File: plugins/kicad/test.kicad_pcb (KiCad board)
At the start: 2 copper layers, 172.7 x 40.6 mm, 2 parts

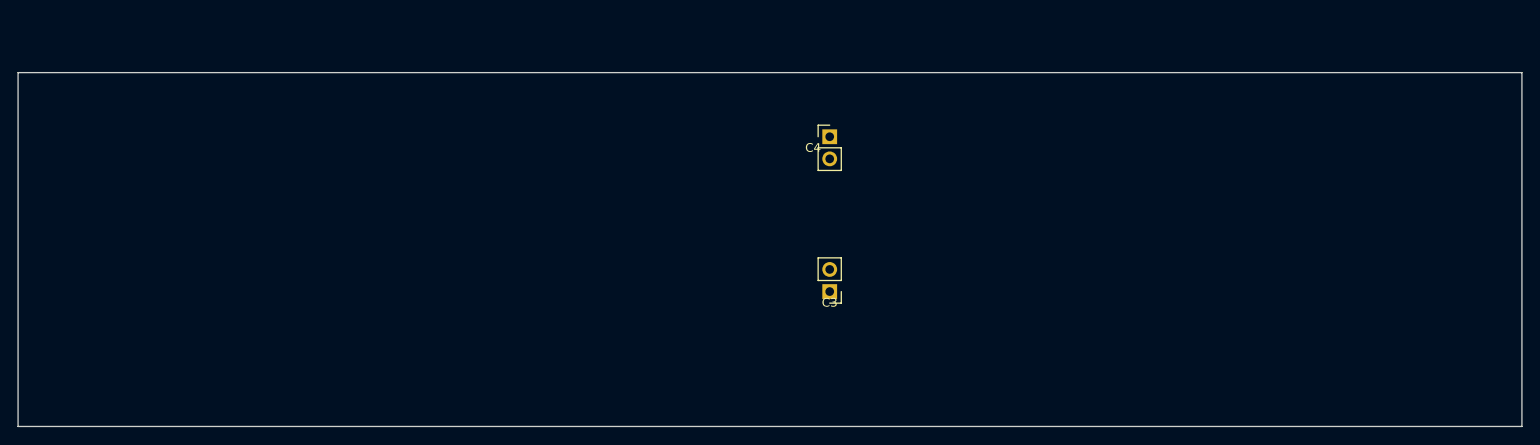
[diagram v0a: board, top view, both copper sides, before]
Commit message: perfectGPT
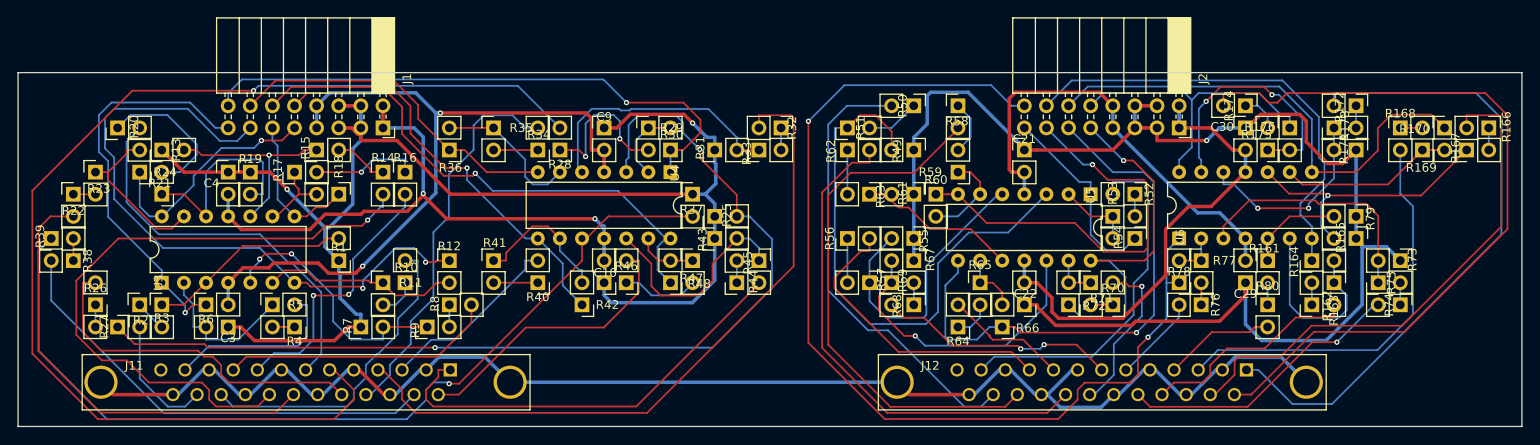
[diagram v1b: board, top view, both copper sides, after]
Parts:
- added C10: 100n, Connector_PinHeader_2.54mm:PinHeader_1x02_P2.54mm_Vertical, F.Cu at (134.6, 215.3)
- added C21: 100n, Connector_PinHeader_2.54mm:PinHeader_1x02_P2.54mm_Vertical, F.Cu at (182.9, 200.0)
- added C22: 100n, Connector_PinHeader_2.54mm:PinHeader_1x02_P2.54mm_Vertical, F.Cu at (182.9, 217.8)
- added C29: 100n, Connector_PinHeader_2.54mm:PinHeader_1x02_P2.54mm_Vertical, F.Cu at (208.3, 215.3)
- added C30: 100n, Connector_PinHeader_2.54mm:PinHeader_1x02_P2.54mm_Vertical, F.Cu at (208.3, 197.5)
- added C9: 100n, Connector_PinHeader_2.54mm:PinHeader_1x02_P2.54mm_Vertical, F.Cu at (134.6, 197.5)
- added J1: CONN_02X08, Connector_PinSocket_2.54mm:PinSocket_2x08_P2.54mm_Horizontal, F.Cu at (109.2, 197.5)
- added J11: DB25_FEMALE, anatalpretty:DB25FD, F.Cu at (100.3, 226.7)
- added J12: DB25_FEMALE, anatalpretty:DB25FD, F.Cu at (191.8, 226.7)
- added J2: CONN_02X08, Connector_PinSocket_2.54mm:PinSocket_2x08_P2.54mm_Horizontal, F.Cu at (200.7, 197.5)
- added R1: 10k, Connector_PinHeader_2.54mm:PinHeader_1x02_P2.54mm_Vertical, F.Cu at (104.1, 212.7)
- added R10: 10k, Connector_PinHeader_2.54mm:PinHeader_1x02_P2.54mm_Vertical, F.Cu at (111.8, 215.3)
- added R11: 10k, Connector_PinHeader_2.54mm:PinHeader_1x02_P2.54mm_Vertical, F.Cu at (109.2, 215.3)
- added R12: 10k, Connector_PinHeader_2.54mm:PinHeader_1x02_P2.54mm_Vertical, F.Cu at (116.8, 212.7)
- added R13: 10k, Connector_PinHeader_2.54mm:PinHeader_1x02_P2.54mm_Vertical, F.Cu at (83.8, 200.0)
- added R14: 10k, Connector_PinHeader_2.54mm:PinHeader_1x02_P2.54mm_Vertical, F.Cu at (109.2, 202.6)
- added R15: 10k, Connector_PinHeader_2.54mm:PinHeader_1x02_P2.54mm_Vertical, F.Cu at (101.6, 200.0)
- added R16: 10k, Connector_PinHeader_2.54mm:PinHeader_1x02_P2.54mm_Vertical, F.Cu at (111.8, 202.6)
- added R161: 10k, Connector_PinHeader_2.54mm:PinHeader_1x02_P2.54mm_Vertical, F.Cu at (210.8, 212.7)
- added R162: 10k, Connector_PinHeader_2.54mm:PinHeader_1x02_P2.54mm_Vertical, F.Cu at (215.9, 217.8)
- added R163: 10k, Connector_PinHeader_2.54mm:PinHeader_1x02_P2.54mm_Vertical, F.Cu at (218.4, 215.3)
- added R164: 10k, Connector_PinHeader_2.54mm:PinHeader_1x02_P2.54mm_Vertical, F.Cu at (215.9, 212.7)
- added R165: 10k, Connector_PinHeader_2.54mm:PinHeader_1x02_P2.54mm_Vertical, F.Cu at (221.0, 210.2)
- added R166: 10k, Connector_PinHeader_2.54mm:PinHeader_1x02_P2.54mm_Vertical, F.Cu at (236.2, 197.5)
- added R167: 10k, Connector_PinHeader_2.54mm:PinHeader_1x02_P2.54mm_Vertical, F.Cu at (233.7, 200.0)
- added R168: 10k, Connector_PinHeader_2.54mm:PinHeader_1x02_P2.54mm_Vertical, F.Cu at (226.1, 197.5)
- added R169: 10k, Connector_PinHeader_2.54mm:PinHeader_1x02_P2.54mm_Vertical, F.Cu at (228.6, 200.0)
- added R17: 10k, Connector_PinHeader_2.54mm:PinHeader_1x02_P2.54mm_Vertical, F.Cu at (99.1, 202.6)
- added R170: 10k, Connector_PinHeader_2.54mm:PinHeader_1x02_P2.54mm_Vertical, F.Cu at (231.1, 197.5)
- added R171: 10k, Connector_PinHeader_2.54mm:PinHeader_1x02_P2.54mm_Vertical, F.Cu at (221.0, 200.0)
- added R172: 10k, Connector_PinHeader_2.54mm:PinHeader_1x02_P2.54mm_Vertical, F.Cu at (221.0, 194.9)
- added R173: 10k, Connector_PinHeader_2.54mm:PinHeader_1x02_P2.54mm_Vertical, F.Cu at (218.4, 197.5)
- added R174: 10k, Connector_PinHeader_2.54mm:PinHeader_1x02_P2.54mm_Vertical, F.Cu at (208.3, 194.9)
- added R175: 10k, Connector_PinHeader_2.54mm:PinHeader_1x02_P2.54mm_Vertical, F.Cu at (210.8, 200.0)
- added R176: 10k, Connector_PinHeader_2.54mm:PinHeader_1x02_P2.54mm_Vertical, F.Cu at (213.4, 197.5)
- added R18: 10k, Connector_PinHeader_2.54mm:PinHeader_1x02_P2.54mm_Vertical, F.Cu at (104.1, 205.1)
- added R19: 10k, Connector_PinHeader_2.54mm:PinHeader_1x02_P2.54mm_Vertical, F.Cu at (94.0, 202.6)
- added R2: 10k, Connector_PinHeader_2.54mm:PinHeader_1x02_P2.54mm_Vertical, F.Cu at (81.3, 217.8)
- added R20: 10k, Connector_PinHeader_2.54mm:PinHeader_1x02_P2.54mm_Vertical, F.Cu at (78.7, 197.5)
- added R21: 10k, Connector_PinHeader_2.54mm:PinHeader_1x02_P2.54mm_Vertical, F.Cu at (83.8, 205.1)
- added R22: 10k, Connector_PinHeader_2.54mm:PinHeader_1x02_P2.54mm_Vertical, F.Cu at (73.7, 205.1)
- added R23: 10k, Connector_PinHeader_2.54mm:PinHeader_1x02_P2.54mm_Vertical, F.Cu at (76.2, 202.6)
- added R24: 10k, Connector_PinHeader_2.54mm:PinHeader_1x02_P2.54mm_Vertical, F.Cu at (81.3, 202.6)
- added R25: 10k, Connector_PinHeader_2.54mm:PinHeader_1x02_P2.54mm_Vertical, F.Cu at (147.3, 207.6)
- added R26: 10k, Connector_PinHeader_2.54mm:PinHeader_1x02_P2.54mm_Vertical, F.Cu at (76.2, 217.8)
- added R27: 10k, Connector_PinHeader_2.54mm:PinHeader_1x02_P2.54mm_Vertical, F.Cu at (78.7, 220.3)
- added R28: 10k, Connector_PinHeader_2.54mm:PinHeader_1x02_P2.54mm_Vertical, F.Cu at (129.5, 200.0)
- added R29: 10k, Connector_PinHeader_2.54mm:PinHeader_1x02_P2.54mm_Vertical, F.Cu at (139.7, 197.5)
- added R3: 10k, Connector_PinHeader_2.54mm:PinHeader_1x02_P2.54mm_Vertical, F.Cu at (83.8, 217.8)
- added R30: 10k, Connector_PinHeader_2.54mm:PinHeader_1x02_P2.54mm_Vertical, F.Cu at (142.2, 200.0)
- added R31: 10k, Connector_PinHeader_2.54mm:PinHeader_1x02_P2.54mm_Vertical, F.Cu at (147.3, 200.0)
- added R32: 10k, Connector_PinHeader_2.54mm:PinHeader_1x02_P2.54mm_Vertical, F.Cu at (154.9, 197.5)
- added R33: 10k, Connector_PinHeader_2.54mm:PinHeader_1x02_P2.54mm_Vertical, F.Cu at (152.4, 200.0)
- added R34: 10k, Connector_PinHeader_2.54mm:PinHeader_1x02_P2.54mm_Vertical, F.Cu at (127.0, 200.0)
- added R35: 10k, Connector_PinHeader_2.54mm:PinHeader_1x02_P2.54mm_Vertical, F.Cu at (121.9, 197.5)
- added R36: 10k, Connector_PinHeader_2.54mm:PinHeader_1x02_P2.54mm_Vertical, F.Cu at (116.8, 200.0)
- added R37: 10k, Connector_PinHeader_2.54mm:PinHeader_1x02_P2.54mm_Vertical, F.Cu at (144.8, 205.1)
- added R38: 10k, Connector_PinHeader_2.54mm:PinHeader_1x02_P2.54mm_Vertical, F.Cu at (73.7, 212.7)
- added R39: 10k, Connector_PinHeader_2.54mm:PinHeader_1x02_P2.54mm_Vertical, F.Cu at (71.1, 210.2)
- added R4: 10k, Connector_PinHeader_2.54mm:PinHeader_1x02_P2.54mm_Vertical, F.Cu at (99.1, 220.3)
- added R40: 10k, Connector_PinHeader_2.54mm:PinHeader_1x02_P2.54mm_Vertical, F.Cu at (127.0, 215.3)
- added R41: 10k, Connector_PinHeader_2.54mm:PinHeader_1x02_P2.54mm_Vertical, F.Cu at (121.9, 212.7)
- added R42: 10k, Connector_PinHeader_2.54mm:PinHeader_1x02_P2.54mm_Vertical, F.Cu at (132.1, 217.8)
- added R43: 10k, Connector_PinHeader_2.54mm:PinHeader_1x02_P2.54mm_Vertical, F.Cu at (147.3, 210.2)
- added R44: 10k, Connector_PinHeader_2.54mm:PinHeader_1x02_P2.54mm_Vertical, F.Cu at (149.9, 215.3)
- added R45: 10k, Connector_PinHeader_2.54mm:PinHeader_1x02_P2.54mm_Vertical, F.Cu at (152.4, 212.7)
- added R46: 10k, Connector_PinHeader_2.54mm:PinHeader_1x02_P2.54mm_Vertical, F.Cu at (137.2, 215.3)
- added R47: 10k, Connector_PinHeader_2.54mm:PinHeader_1x02_P2.54mm_Vertical, F.Cu at (144.8, 212.7)
- added R48: 10k, Connector_PinHeader_2.54mm:PinHeader_1x02_P2.54mm_Vertical, F.Cu at (142.2, 215.3)
- added R49: 10k, Connector_PinHeader_2.54mm:PinHeader_1x02_P2.54mm_Vertical, F.Cu at (170.2, 200.0)
- added R5: 10k, Connector_PinHeader_2.54mm:PinHeader_1x02_P2.54mm_Vertical, F.Cu at (96.5, 217.8)
- added R50: 10k, Connector_PinHeader_2.54mm:PinHeader_1x02_P2.54mm_Vertical, F.Cu at (170.2, 194.9)
- added R51: 10k, Connector_PinHeader_2.54mm:PinHeader_1x02_P2.54mm_Vertical, F.Cu at (162.6, 197.5)
- added R52: 10k, Connector_PinHeader_2.54mm:PinHeader_1x02_P2.54mm_Vertical, F.Cu at (195.6, 205.1)
- added R53: 10k, Connector_PinHeader_2.54mm:PinHeader_1x02_P2.54mm_Vertical, F.Cu at (193.0, 207.6)
- added R54: 10k, Connector_PinHeader_2.54mm:PinHeader_1x02_P2.54mm_Vertical, F.Cu at (195.6, 210.2)
- added R55: 10k, Connector_PinHeader_2.54mm:PinHeader_1x02_P2.54mm_Vertical, F.Cu at (170.2, 210.2)
- added R56: 10k, Connector_PinHeader_2.54mm:PinHeader_1x02_P2.54mm_Vertical, F.Cu at (162.6, 210.2)
- added R57: 10k, Connector_PinHeader_2.54mm:PinHeader_1x02_P2.54mm_Vertical, F.Cu at (165.1, 215.3)
- added R58: 10k, Connector_PinHeader_2.54mm:PinHeader_1x02_P2.54mm_Vertical, F.Cu at (175.3, 194.9)
- added R59: 10k, Connector_PinHeader_2.54mm:PinHeader_1x02_P2.54mm_Vertical, F.Cu at (175.3, 202.6)
- added R6: 10k, Connector_PinHeader_2.54mm:PinHeader_1x02_P2.54mm_Vertical, F.Cu at (88.9, 217.8)
- added R60: 10k, Connector_PinHeader_2.54mm:PinHeader_1x02_P2.54mm_Vertical, F.Cu at (172.7, 205.1)
- added R61: 10k, Connector_PinHeader_2.54mm:PinHeader_1x02_P2.54mm_Vertical, F.Cu at (170.2, 205.1)
- added R62: 10k, Connector_PinHeader_2.54mm:PinHeader_1x02_P2.54mm_Vertical, F.Cu at (162.6, 200.0)
- added R63: 10k, Connector_PinHeader_2.54mm:PinHeader_1x02_P2.54mm_Vertical, F.Cu at (165.1, 205.1)
- added R64: 10k, Connector_PinHeader_2.54mm:PinHeader_1x02_P2.54mm_Vertical, F.Cu at (175.3, 220.3)
- added R65: 10k, Connector_PinHeader_2.54mm:PinHeader_1x02_P2.54mm_Vertical, F.Cu at (177.8, 215.3)
- added R66: 10k, Connector_PinHeader_2.54mm:PinHeader_1x02_P2.54mm_Vertical, F.Cu at (180.3, 220.3)
- added R67: 10k, Connector_PinHeader_2.54mm:PinHeader_1x02_P2.54mm_Vertical, F.Cu at (170.2, 212.7)
- added R68: 10k, Connector_PinHeader_2.54mm:PinHeader_1x02_P2.54mm_Vertical, F.Cu at (170.2, 217.8)
- added R69: 10k, Connector_PinHeader_2.54mm:PinHeader_1x02_P2.54mm_Vertical, F.Cu at (167.6, 215.3)
- added R7: 10k, Connector_PinHeader_2.54mm:PinHeader_1x02_P2.54mm_Vertical, F.Cu at (106.7, 220.3)
- added R70: 10k, Connector_PinHeader_2.54mm:PinHeader_1x02_P2.54mm_Vertical, F.Cu at (193.0, 217.8)
- added R71: 10k, Connector_PinHeader_2.54mm:PinHeader_1x02_P2.54mm_Vertical, F.Cu at (190.5, 215.3)
- added R72: 10k, Connector_PinHeader_2.54mm:PinHeader_1x02_P2.54mm_Vertical, F.Cu at (188.0, 217.8)
- added R73: 10k, Connector_PinHeader_2.54mm:PinHeader_1x02_P2.54mm_Vertical, F.Cu at (226.1, 212.7)
- added R74: 10k, Connector_PinHeader_2.54mm:PinHeader_1x02_P2.54mm_Vertical, F.Cu at (226.1, 217.8)
- added R75: 10k, Connector_PinHeader_2.54mm:PinHeader_1x02_P2.54mm_Vertical, F.Cu at (223.5, 215.3)
- added R76: 10k, Connector_PinHeader_2.54mm:PinHeader_1x02_P2.54mm_Vertical, F.Cu at (203.2, 217.8)
- added R77: 10k, Connector_PinHeader_2.54mm:PinHeader_1x02_P2.54mm_Vertical, F.Cu at (203.2, 212.7)
- added R78: 10k, Connector_PinHeader_2.54mm:PinHeader_1x02_P2.54mm_Vertical, F.Cu at (200.7, 215.3)
- added R79: 10k, Connector_PinHeader_2.54mm:PinHeader_1x02_P2.54mm_Vertical, F.Cu at (221.0, 207.6)
- added R8: 10k, Connector_PinHeader_2.54mm:PinHeader_1x02_P2.54mm_Vertical, F.Cu at (116.8, 217.8)
- added R80: 10k, Connector_PinHeader_2.54mm:PinHeader_1x02_P2.54mm_Vertical, F.Cu at (210.8, 217.8)
- added R9: 10k, Connector_PinHeader_2.54mm:PinHeader_1x02_P2.54mm_Vertical, F.Cu at (114.3, 220.3)
- added U3: OPA4340D, Package_DIP:DIP-14_W7.62mm, F.Cu at (83.8, 215.3)
- added U4: OPA4340D, Package_DIP:DIP-14_W7.62mm, F.Cu at (142.2, 202.6)
- added U5: OPA4340D, Package_DIP:DIP-14_W7.62mm, F.Cu at (190.5, 205.1)
- added U6: OPA4340D, Package_DIP:DIP-14_W7.62mm, F.Cu at (200.7, 210.2)
- moved C3 69.2 mm to (91.4, 220.3)
- moved C4 69.2 mm to (91.4, 202.6)
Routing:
- net GND: track 0.00 -> 322.9 mm, vias 0 -> 3
- net GNDPWR: track 0.00 -> 163.2 mm
- net +12V: track 0.00 -> 135.4 mm, vias 0 -> 2
- net /din5-: track 0.00 -> 132.1 mm, vias 0 -> 1
- net -12V: track 0.00 -> 122.1 mm, vias 0 -> 2
- net /quad3/out1: track 0.00 -> 116.2 mm, vias 0 -> 2
- net Net-(R25-Pad2): track 0.00 -> 115.7 mm, vias 0 -> 2
- net Net-(R37-Pad2): track 0.00 -> 103.8 mm, vias 0 -> 1
- net /din16-: track 0.00 -> 88.4 mm
- net /din6+: track 0.00 -> 80.0 mm
- net /quad2/out2: track 0.00 -> 75.2 mm, vias 0 -> 2
- net /din16+: track 0.00 -> 74.2 mm
- net /din3+: track 0.00 -> 73.2 mm, vias 0 -> 1
- net /quad1/out1: track 0.00 -> 66.6 mm, vias 0 -> 1
- net Net-(R49-Pad2): track 0.00 -> 63.9 mm
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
